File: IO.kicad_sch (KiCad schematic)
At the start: 5 parts, among them J1 conn_USB-A-(UE27AC54100), U12 AS5F32G04SNDA-08LIN(mémoire), U13 AS5F32G04SNDA-08LIN(mémoire)

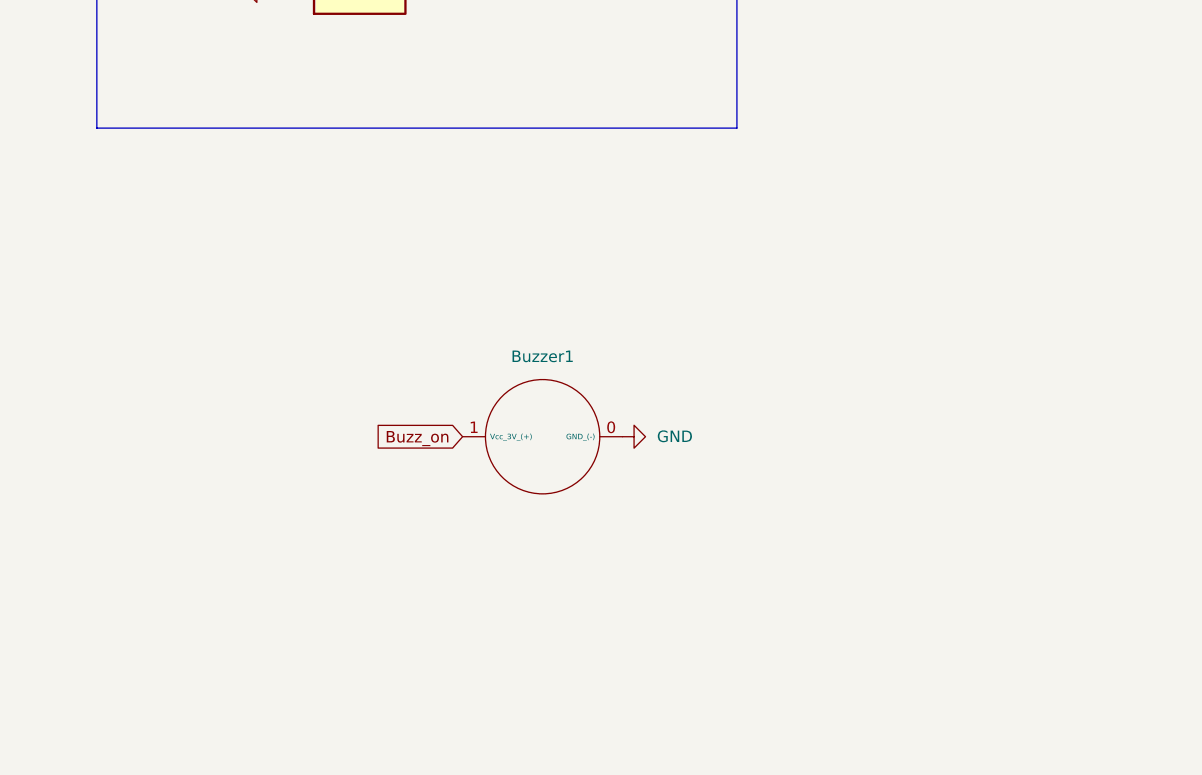
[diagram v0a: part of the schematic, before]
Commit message: Début PCB
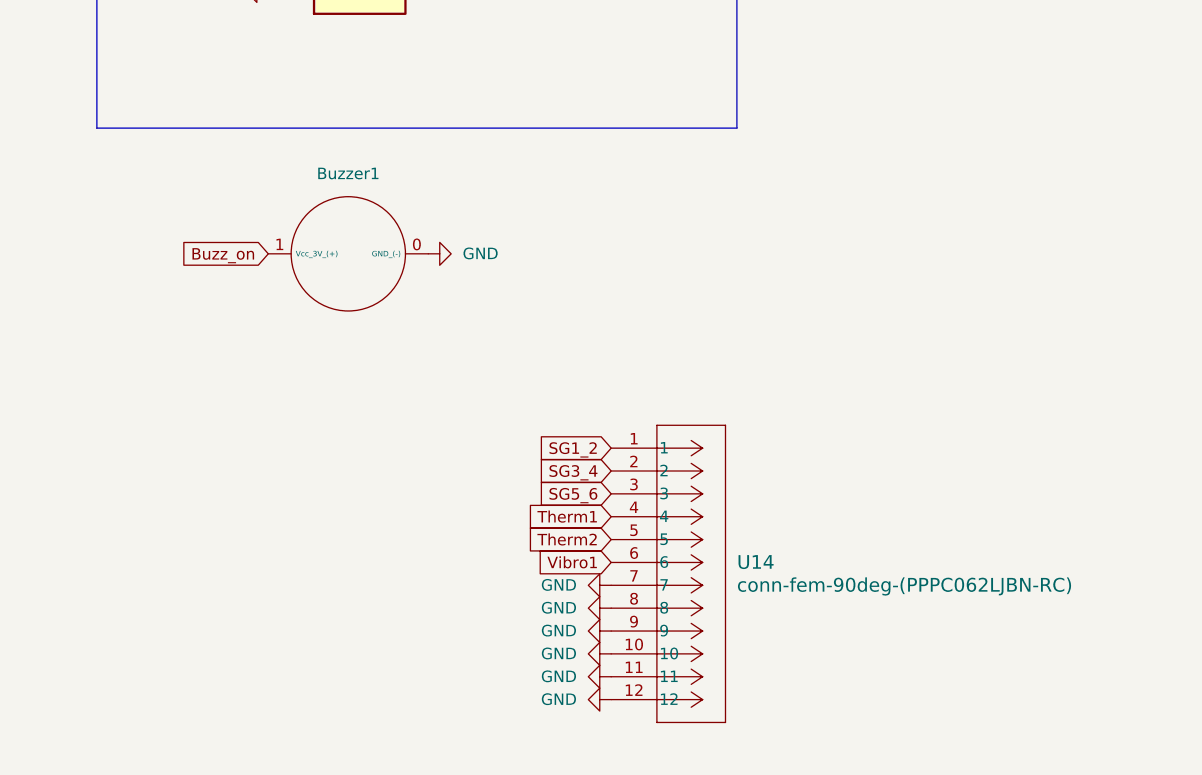
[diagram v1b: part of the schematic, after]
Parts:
- added U14: conn-fem-90deg-(PPPC062LJBN-RC), GAUL-Empreintes:conn-90deg-(CONN_PPPC062LJBN-RC_SUL), symbol GAUL-Symboles:conn-fem-90deg-(PPPC062LJBN-RC)
- Buzzer1: footprint (none) -> GAUL-Empreintes:buzzer-(IE092503-1)
- J1: footprint UE27AC54100:AMPHENOL_UE27AC54100 -> GAUL-Empreintes:conn-usbA-(AMPHENOL_UE27AC54100)
- Programming_pins1: footprint (none) -> GAUL-Empreintes:conn-swd5pin-(CONN5_1LFBN-RC_SUL)
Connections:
- net GND: now also U14.10, U14.11, U14.12, U14.7, U14.8, U14.9
- new net SG1_2: U14.1
- new net SG3_4: U14.2
- new net SG5_6: U14.3
- new net Therm1: U14.4
- new net Therm2: U14.5
- new net Vibro1: U14.6
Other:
- moved on the sheet: Buzzer1
